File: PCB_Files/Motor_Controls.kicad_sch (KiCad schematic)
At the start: 14 parts, among them M1 Front_Right_Motor, M2 Rear_Right_Motor, M3 Front_Left_Motor, M4 Rear_Left_Motor, U2 TB6612FNG, U3 TB6612FNG

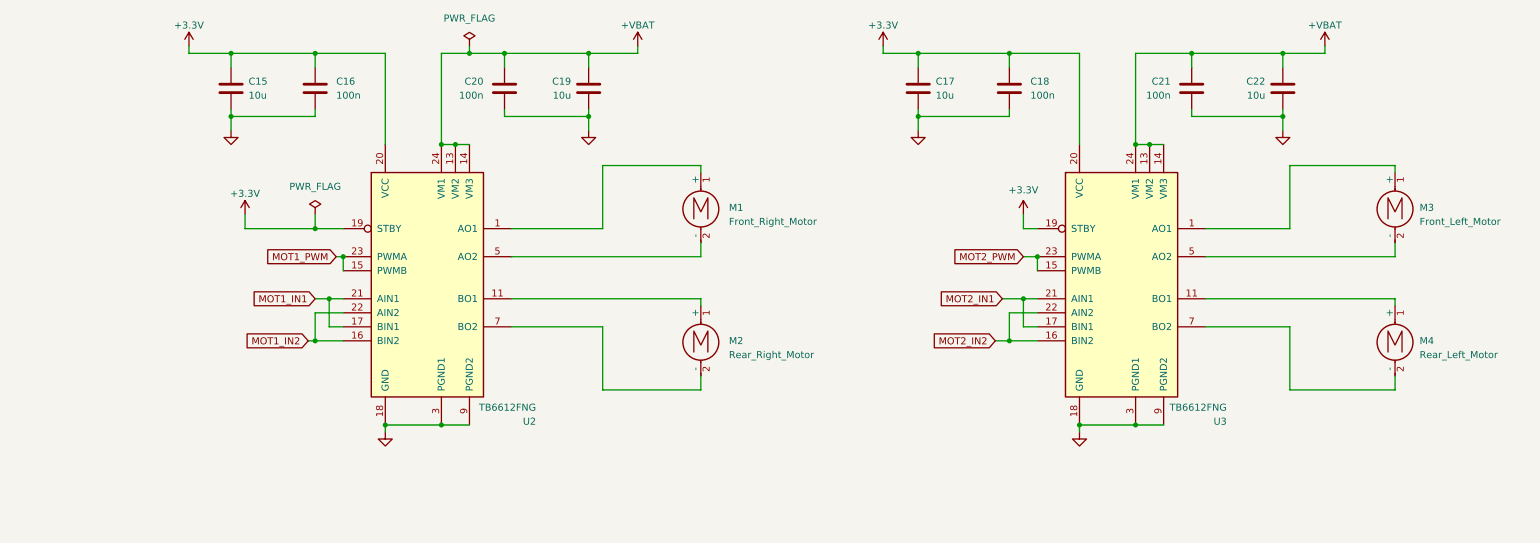
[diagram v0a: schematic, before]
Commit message: General schematic clean up and footprint allocation.
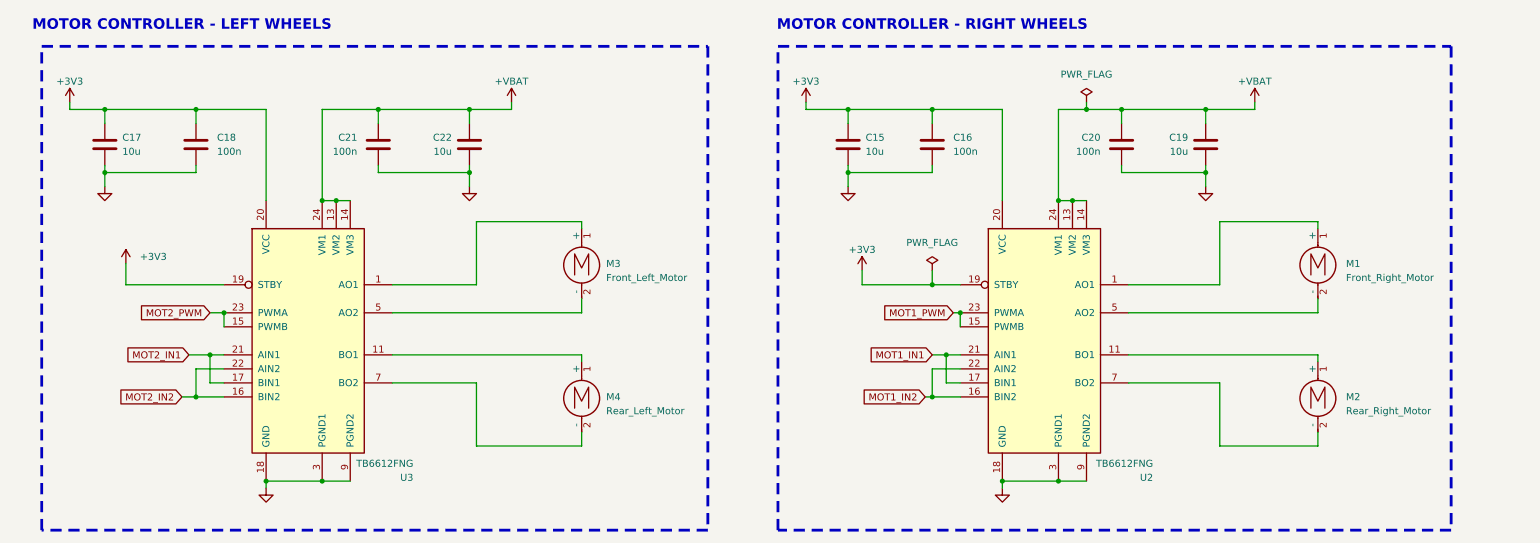
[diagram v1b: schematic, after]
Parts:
- C15, C16, C17, C18, C19, C20, C21, C22: footprint (none) -> Capacitor_SMD:C_0603_1608Metric
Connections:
- net +3.3V renamed +3V3
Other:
- note added: "MOTOR CONTROLLER - LEFT WHEELS"
- note added: "MOTOR CONTROLLER - RIGHT WHEELS"
- moved on the sheet: C15, C16, C17, C18, C19, C20, C21, C22, M1, M2, M3, M4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
